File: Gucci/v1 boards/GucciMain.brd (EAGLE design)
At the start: 43.2 x 46.7 mm, 15 parts

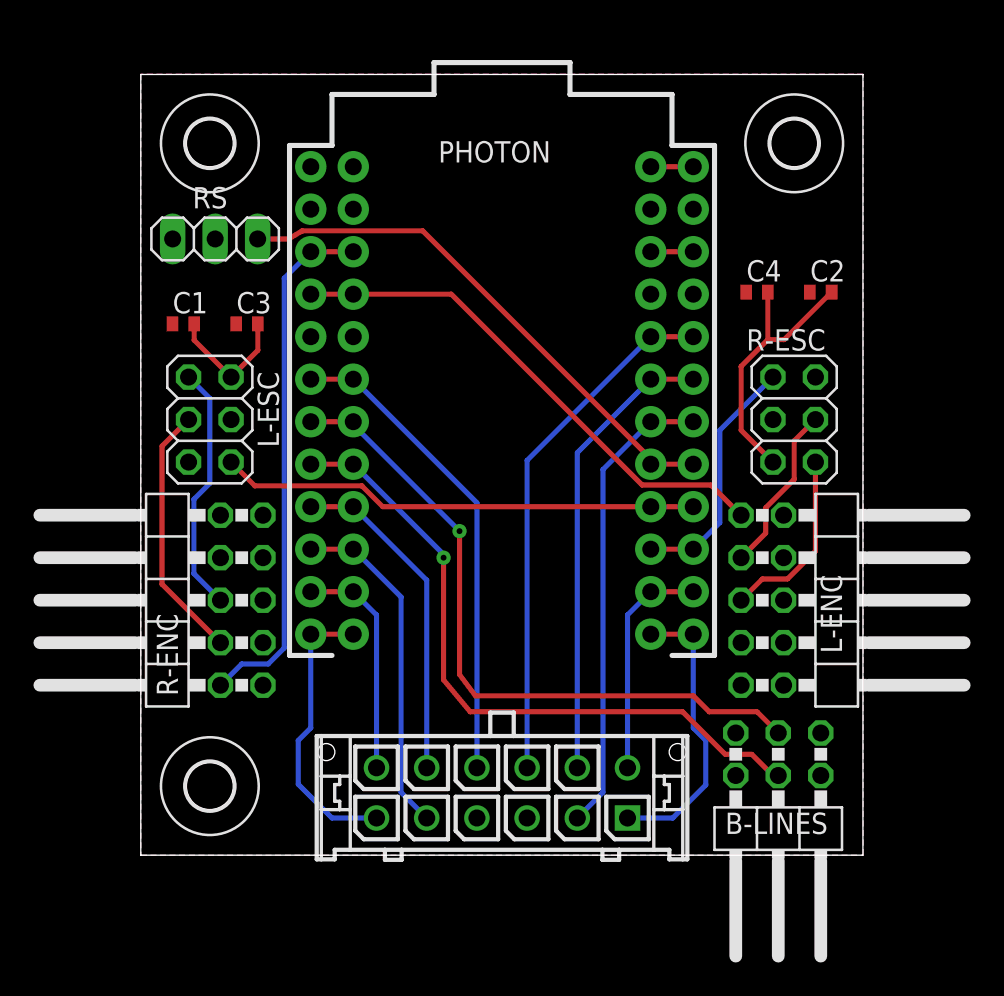
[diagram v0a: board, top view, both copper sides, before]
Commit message: Add files via upload
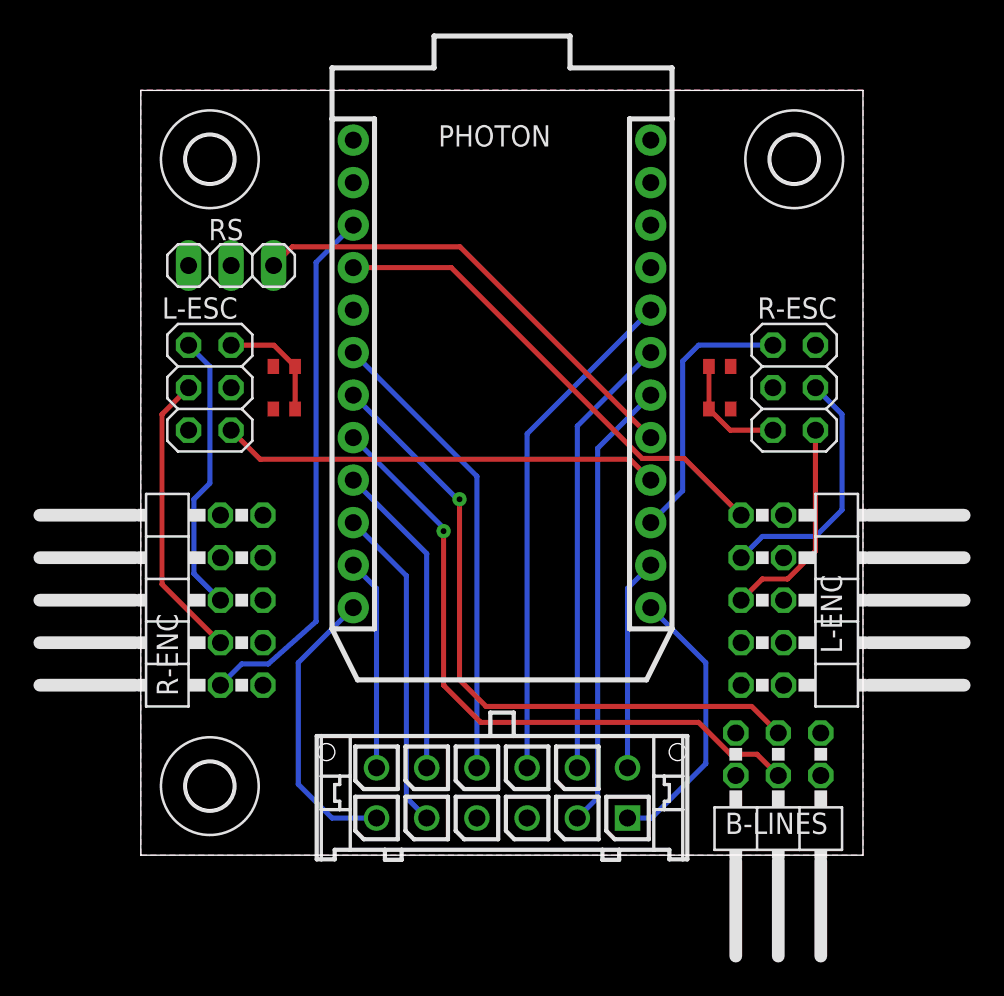
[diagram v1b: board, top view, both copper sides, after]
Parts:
- PHOTON: value (none) -> PHOTON; device Spark:PHOTON_STACKABLE -> Particle:PHOTON
- moved C2 9.23 mm to (34.6, 26.7), turned to 180 degrees
- moved C1 6.55 mm to (8.57, 29.2)
- moved C3 5.54 mm to (8.57, 26.7)
- moved C4 4.97 mm to (34.6, 29.2), turned to 180 degrees
- moved L-ESC 1.91 mm to (4.13, 27.9)
- moved R-ESC 1.91 mm to (39.1, 27.9)
- moved RS 1.85 mm to (5.40, 35.2)
- moved PHOTON 1.59 mm to (11.4, 10.5)
- moved U$3 0.95 mm to (4.13, 41.6)
- moved U$4 0.95 mm to (39.1, 41.6)
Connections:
- net 3V3: no longer PHOTON.#24
- net BL: no longer PHOTON.@8
- net BR: no longer PHOTON.@7
- net FL: no longer PHOTON.@10
- net FR: no longer PHOTON.@9
- net GND: no longer PHOTON.#21, PHOTON.@2
- net I1: no longer PHOTON.@4
- net I2: no longer PHOTON.@3
- net L-CONTROL: no longer PHOTON.#15
- net R-CONTROL: no longer PHOTON.#16
- net RS-OUT: no longer PHOTON.#17
- net SCL: no longer PHOTON.#14
- net SDA: no longer PHOTON.#13
- net SHDN1: no longer PHOTON.@12
- net SHDN2: no longer PHOTON.@11
- net SHDN3: no longer PHOTON.@6
- net SHDN4: no longer PHOTON.#18
- net SHDN5: no longer PHOTON.#19
- net SHDN6: no longer PHOTON.#20
- net VBAT: no longer PHOTON.#22
- net VCC: no longer PHOTON.@1
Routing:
- net GND: track 24.5 -> 13.8 mm
- net B1: track 10.1 -> 15.2 mm
- net RS-OUT: track 32.3 -> 27.7 mm
- net VBAT: track 2.54 -> 0.00 mm
- net 3V3: track 2.54 -> 0.00 mm
- net R-CONTROL: track 28.7 -> 26.3 mm
- net A2: track 14.9 -> 16.8 mm
- net B2: track 15.4 -> 17.3 mm
- net A1: track 11.0 -> 12.9 mm
- net I1: track 31.2 -> 29.3 mm
- net L-CONTROL: track 14.8 -> 16.2 mm
- net SHDN6: track 31.4 -> 30.4 mm
- net SHDN4: track 28.0 -> 27.1 mm
- net SHDN5: track 27.6 -> 26.6 mm
- net SHDN3: track 28.8 -> 27.9 mm
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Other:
- board size 43.2 x 46.7 mm -> 43.2 x 45.7 mm
